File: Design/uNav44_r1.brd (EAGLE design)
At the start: 39.9 x 39.9 mm, 74 parts, among them IC1 DSPIC33FJ128MC, IC2 24LC024, IC3 AP3417CK-3.3TRG1, IC4 AP6503SP-13, U1 MCP6G01T-E/OT, U2 MCP6G01T-E/OT, U3 MCP6G01T-E/OT, U4 MCP6G01T-E/OT

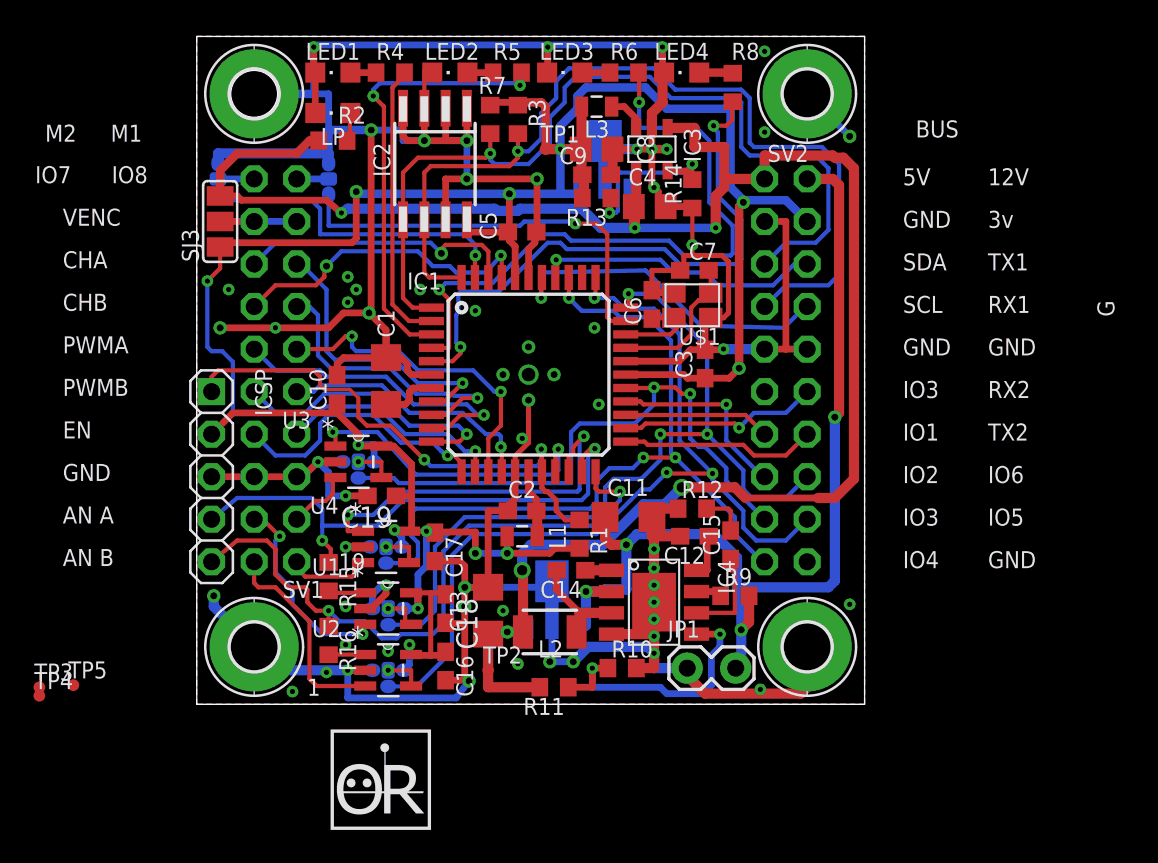
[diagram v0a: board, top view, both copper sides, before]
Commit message: uNAV44 finished.
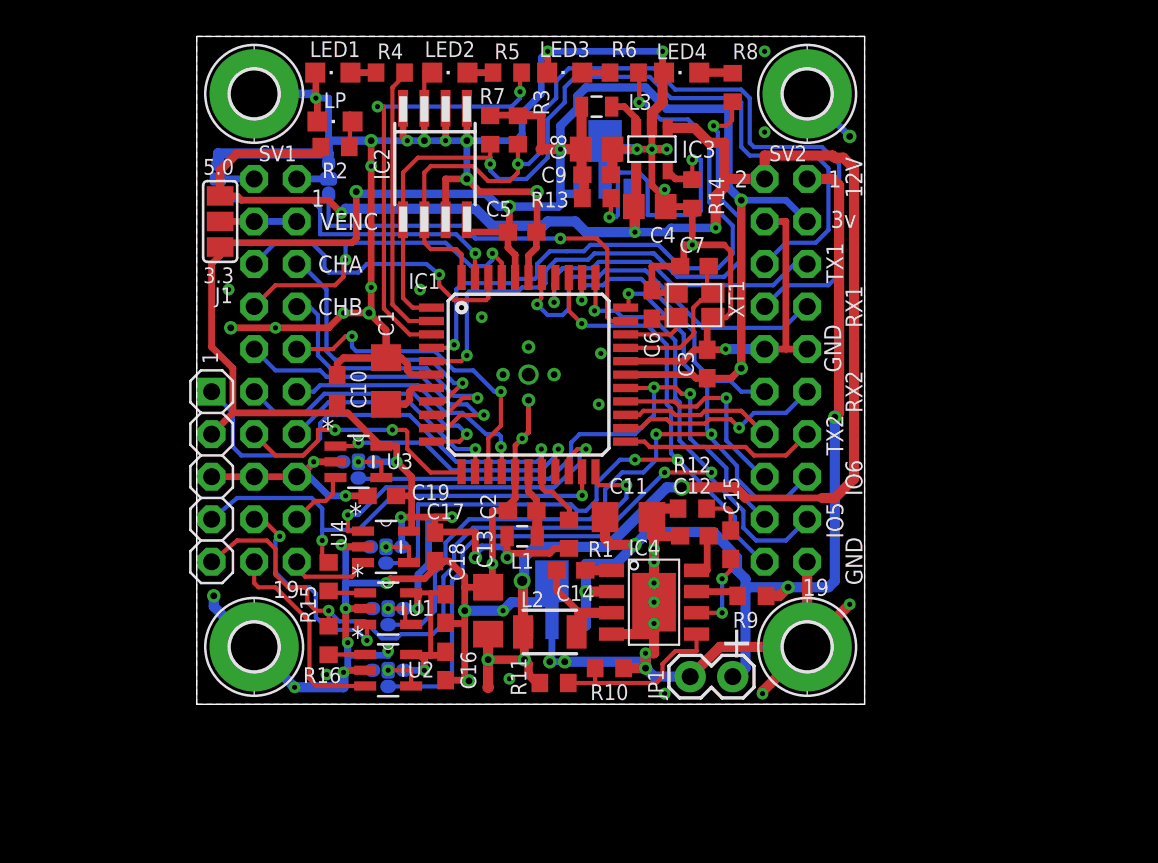
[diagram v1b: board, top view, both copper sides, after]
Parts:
- removed TP3, TP4, TP5: PTR1TP07R, testpad:TP07R
- removed U$1: (no value), OfficineRobotiche:CTS_32X25
- added XT1: (no value), OfficineRobotiche:CTS_32X25
- JP1: value M02LOCK -> M02PTH; device SparkFun-Connectors:1X02_LOCK -> SparkFun-Connectors:1X02
- moved TP2 1.02 mm to (14.0, -2.41)
- moved R9 1.02 mm to (29.7, 3.05)
- moved R10 0.76 mm to (21.2, -1.27)
- moved R1 0.64 mm to (18.8, 6.73)
- moved R3 0.63 mm to (15.7, 30.9)
- moved R7 0.63 mm to (14.1, 30.9)
- moved LP 0.52 mm to (4.83, 31.4)
- moved JP1 0.51 mm to (26.0, -1.78)
- moved R2 0.40 mm to (4.83, 29.8)
- moved C7 0.25 mm to (26.3, 22.7)
- moved TP1 0.25 mm to (17.1, 29.7)
- moved R11 0.25 mm to (17.9, -2.16)
- moved C3 0.13 mm to (27.1, 16.9)
- renumbered JMP5 to J6, JMP6 to J7, JP2 to J2, JP3 to J3, JP4 to J4, JP5 to J5, SJ3 to J1
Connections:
- removed net HALT: IC1.35
- new net IO0: IC1.35, SV2.12
- net GND: now also XT1.2, XT1.4; no longer U$1.2, U$1.4
- net N$2: now also XT1.1; no longer U$1.1
- net N$3: now also XT1.3; no longer U$1.3
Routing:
- net IO0: track 0.00 -> 17.2 mm, vias 0 -> 1
- net N$7: track 11.1 -> 18.0 mm
- net N$9: track 16.9 -> 11.4 mm, vias 2 -> 0
- net TX1: track 17.2 -> 21.1 mm
- net GND: track 302.3 -> 305.8 mm, vias 61 -> 64
- net ANA2/PGD: track 32.3 -> 28.9 mm
- net +5V: track 122.2 -> 124.4 mm, vias 6 -> 7
- net ANB1: track 22.1 -> 20.1 mm
- net ANA1: track 18.3 -> 16.3 mm
- net RX1: track 20.5 -> 22.1 mm
- net CHA2: track 16.8 -> 18.4 mm
- net LD3: track 39.5 -> 38.2 mm
- net ANA2: track 12.2 -> 13.4 mm
- net SCL: track 54.2 -> 55.3 mm
- net IO3: track 36.2 -> 35.1 mm
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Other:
- board text added: "2"
- board text added: "3.3"
- board text added: "5.0"
- board text removed: "5V"
- board text removed: "AN A"
- board text removed: "AN B"
- board text removed: "BUS"
- board text removed: "M1"
- board text removed: "M2"
